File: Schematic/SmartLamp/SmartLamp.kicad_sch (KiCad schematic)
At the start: 7 parts, among them SW1 SW_SPST, SW2 SW_Push, U3 ESP32-DEVKIT-V1

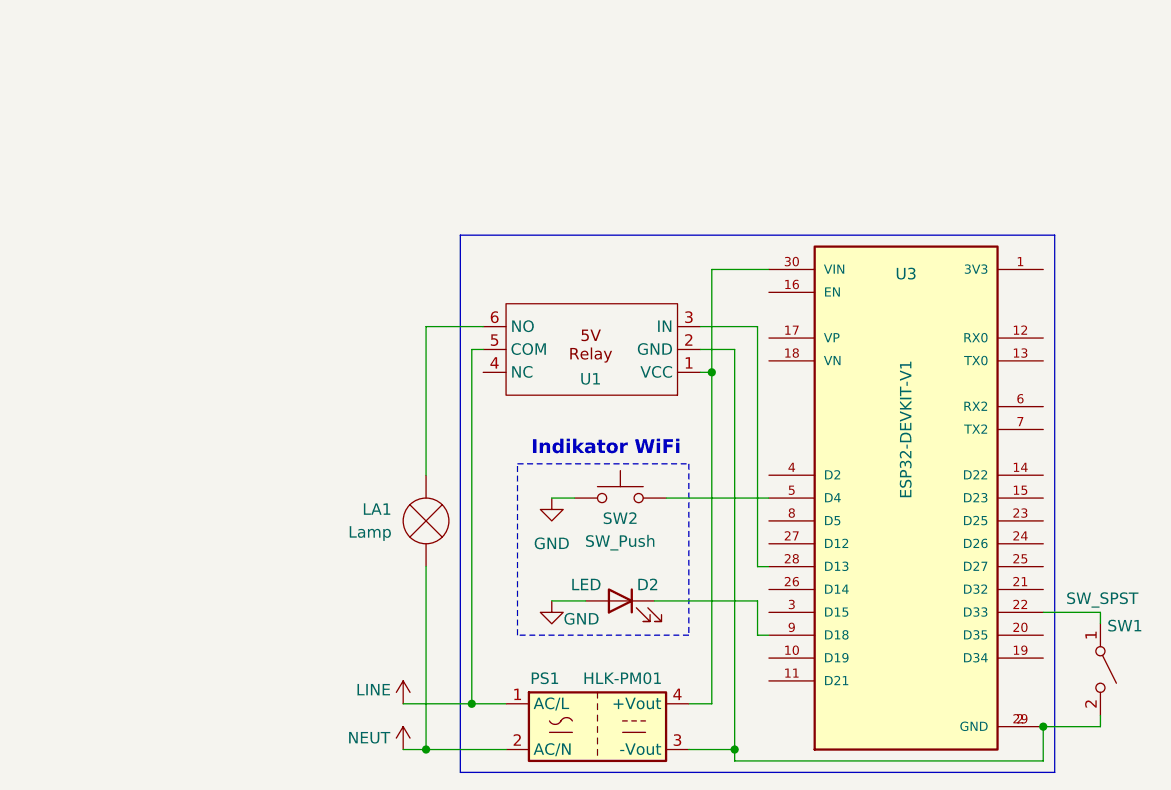
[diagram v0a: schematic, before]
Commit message: update readme
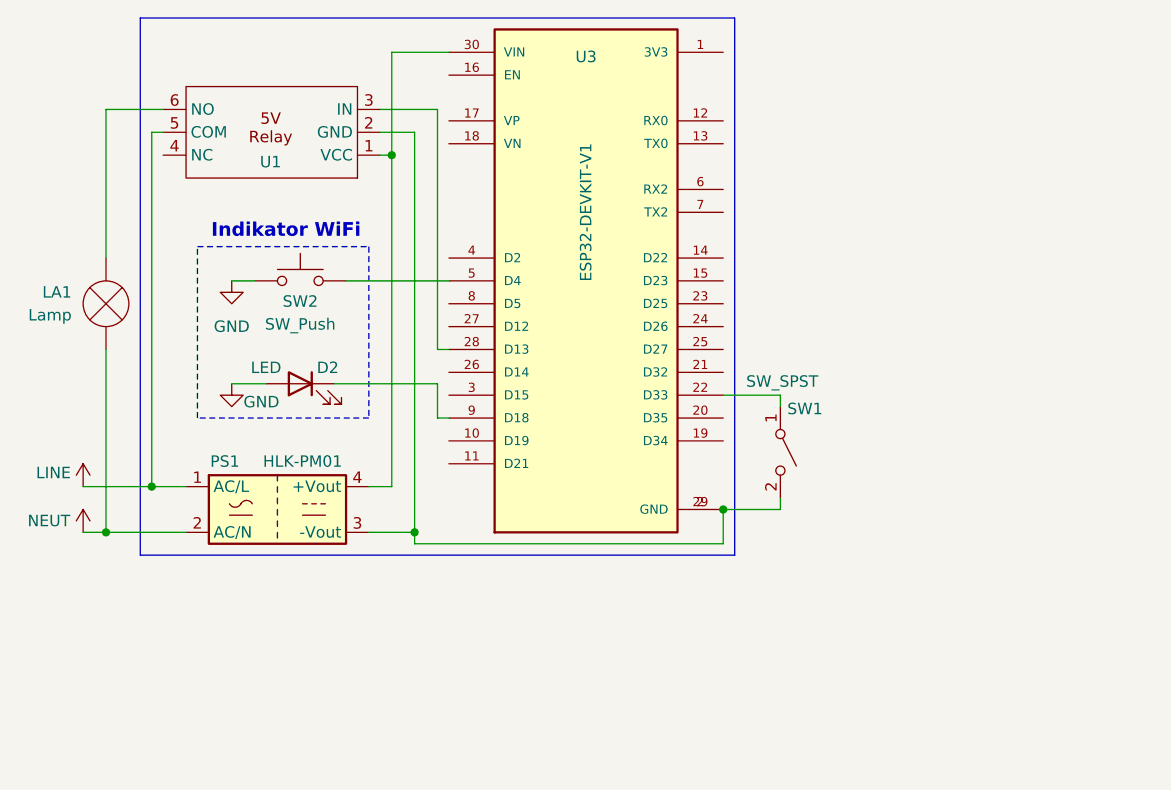
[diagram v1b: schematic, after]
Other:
- title: (none) -> Smart Lamp
- moved on the sheet: D2, LA1, PS1, SW1, SW2, U1, U3
